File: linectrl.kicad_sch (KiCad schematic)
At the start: 22 parts, among them K1 Relay_SPST-NO, K2 Relay_SPDT, Q1 PMOS, Q2 PMOS, T1 Transformer_1P_1S, U5 LM358

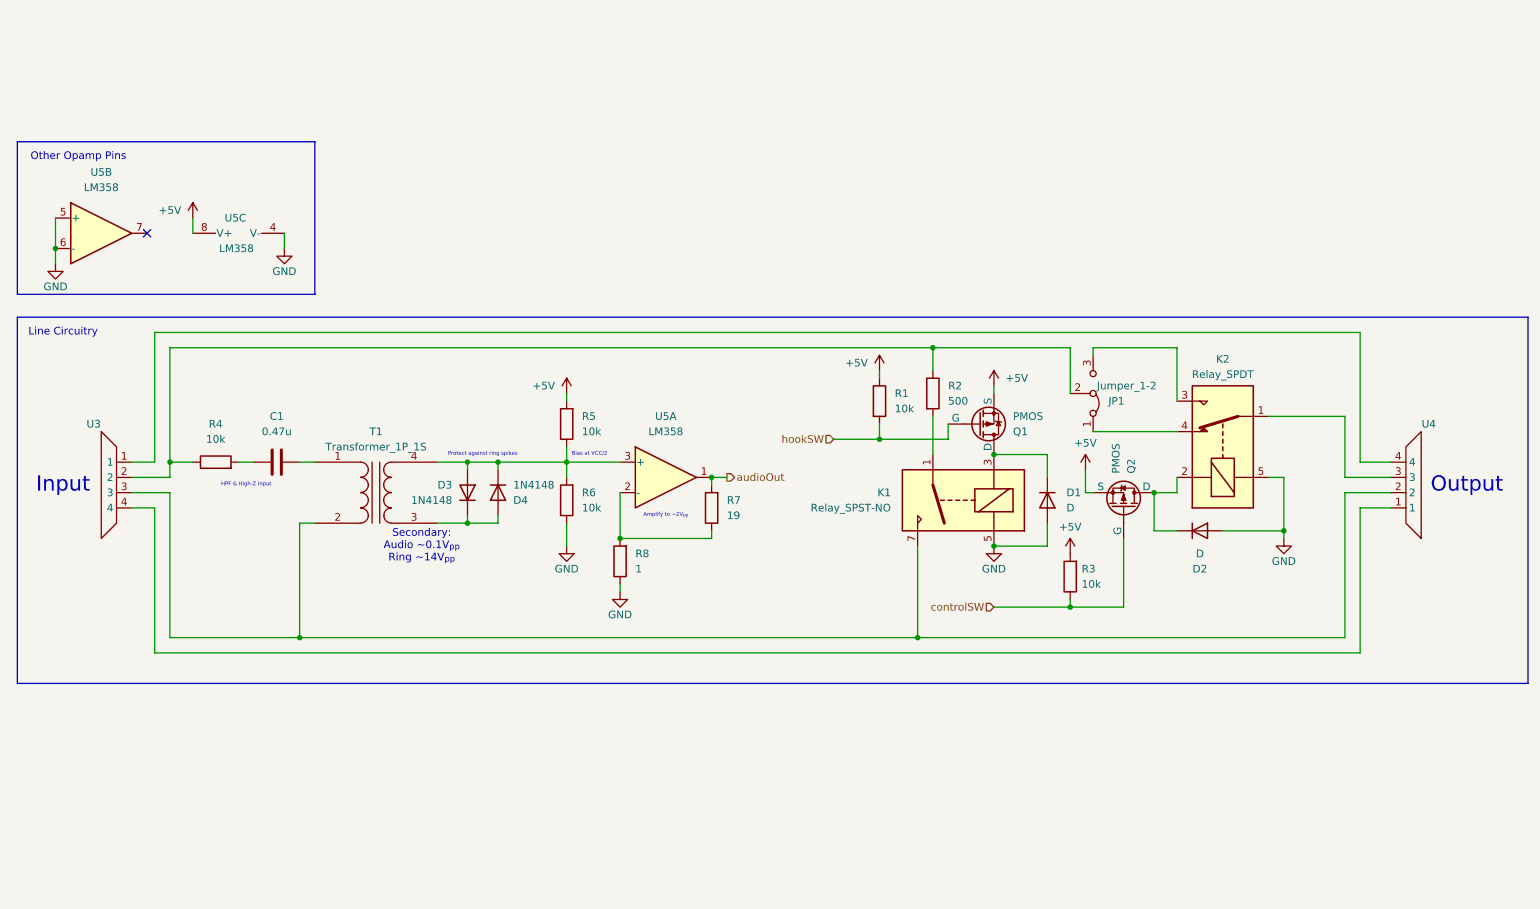
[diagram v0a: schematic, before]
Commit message: finish linectrl implementation
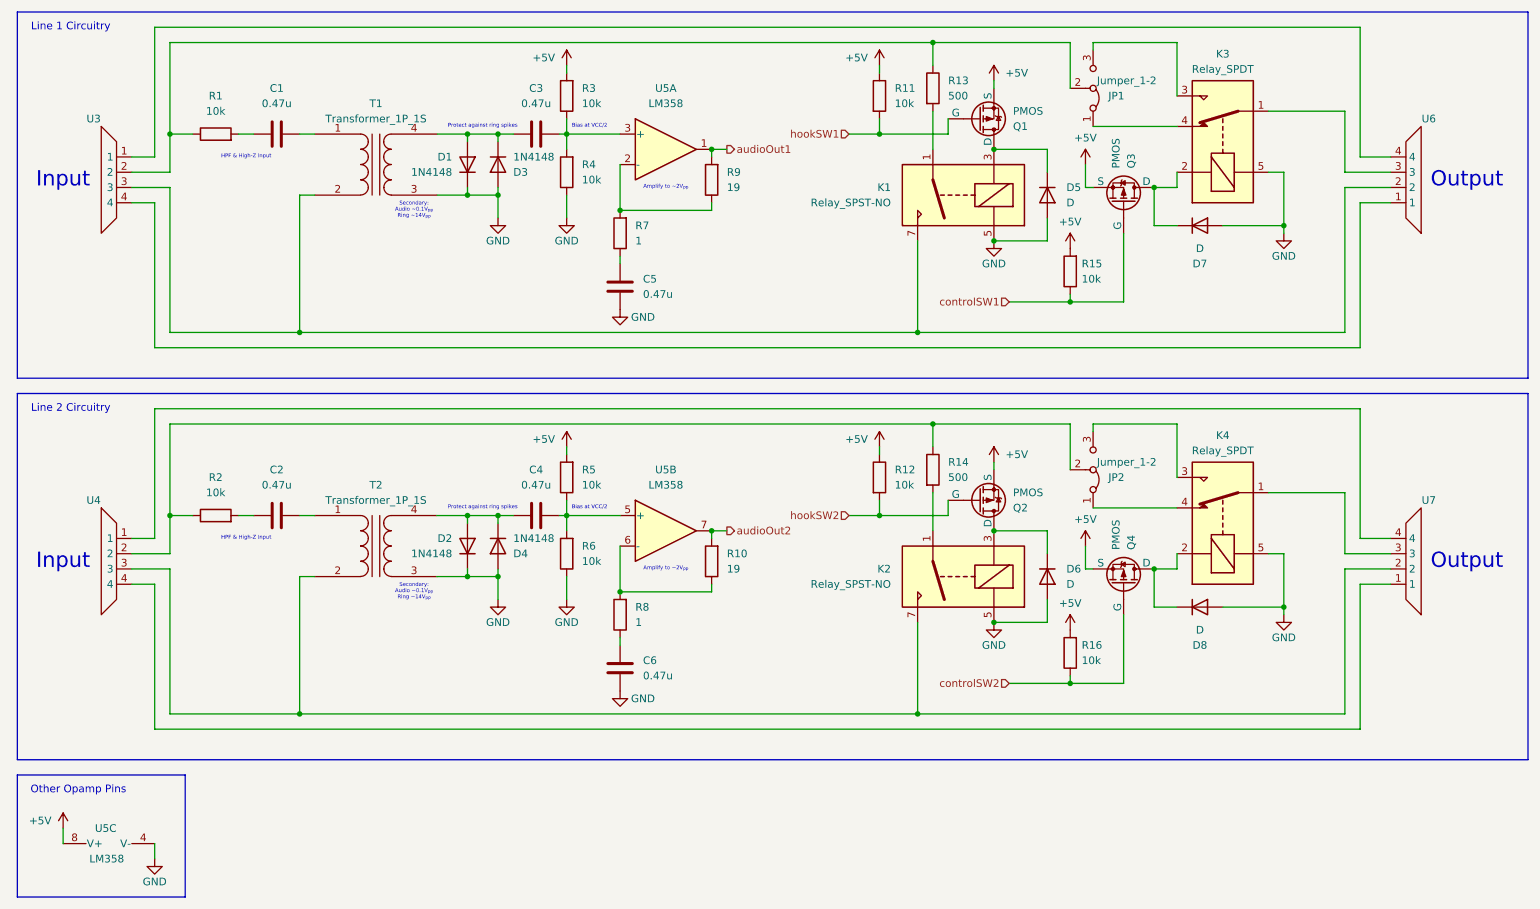
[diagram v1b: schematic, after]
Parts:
- added C2, C3, C4, C5, C6: 0.47u, symbol Device:C
- added D2, D4: 1N4148, Diode_THT:D_DO-35_SOD27_P7.62mm_Horizontal, symbol Diode:1N4148
- added D6, D8: D, Diode_THT:D_A-405_P12.70mm_Horizontal, symbol Device:D
- added JP2: Jumper_1-2, Jumper:SolderJumper-3_P1.3mm_Bridged2Bar12_RoundedPad1.0x1.5mm, symbol Jumper:Jumper_3_Bridged12
- added K2: Relay_SPST-NO, Relay_THT:Relay_SPST_StandexMeder_SIL_Form1A, symbol Relay:Relay_SPST-NO
- added K4: Relay_SPDT, Phones:K_AZ943-1C_AMZ, symbol Relay:Relay_SPDT
- added Q2, Q4: PMOS, Package_TO_SOT_THT:TO-92_HandSolder, symbol Simulation_SPICE:PMOS
- added R10: 19, symbol Device:R
- added R12, R16: 10k, Resistor_THT:R_Axial_DIN0207_L6.3mm_D2.5mm_P10.16mm_Horizontal, symbol Device:R
- added R14: 500, Resistor_THT:R_Axial_DIN0207_L6.3mm_D2.5mm_P10.16mm_Horizontal, symbol Device:R
- added R2, R5, R6: 10k, symbol Device:R
- added R8: 1, symbol Device:R
- added T2: Transformer_1P_1S, symbol Device:Transformer_1P_1S
- added U4, U7: (no value), symbol Phones:4C_Connector
- renumbered D3 to D1, D4 to D3, D1 to D5, D2 to D7, K2 to K3, Q2 to Q3, R4 to R1, R1 to R11, R2 to R13, R3 to R15, R5 to R3, R6 to R4, R8 to R7, R7 to R9, U4 to U6
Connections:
- net +5V: now also Q2.3 (S), Q4.3 (S), R12.1, R16.2, R5.2
- net GND: now also D1.1 (K), D3.2 (A), T1.3 (SA), C5.1, C6.1, D2.1 (K), D4.2 (A), D6.2 (A), D8.2 (A), K2.5, K4.5, R6.1, T2.3 (SA); no longer R7.1, U5.5 (+), U5.6 (-)
- net audioOut2: now reaches U5.7
- net audioOut2: now also R10.2
- net at D1.2 (A), D3.1 (K), T1.4 (SB): now also C3.1; no longer R3.1, R4.2, U5.3 (+)
- net audioOut renamed audioOut1
- net controlSW renamed controlSW1
- net hookSW renamed hookSW1
- new net: JP2.2 (C), R14.1, R2.1, U4.2
- new net: C2.1, R2.2
- new net: C4.2, R5.1, R6.2, U5.5 (+)
- new net: R10.1, R8.2, U5.6 (-)
- new net: JP2.1 (A), K4.4
- new net: JP2.3 (B), K4.3
- new net: K2.1, R14.2
- new net: D6.1 (K), K2.3, Q2.1 (D)
- new net: K2.7, T2.2 (AB), U4.3, U7.2
- new net: C2.2, T2.1 (AA)
- new net: C4.1, D2.2 (A), D4.1 (K), T2.4 (SB)
- new net: C6.2, R8.1
- new net: D8.1 (K), K4.2, Q4.1 (D)
- new net: C5.2, R7.1
- new net: C3.2, R3.1, R4.2, U5.3 (+)
- new net: U4.4, U7.1
- new net: K4.1, U7.3
- new net: U4.1, U7.4
- new net controlSW2: Q4.2 (G), R16.1
- new net hookSW2: Q2.2 (G), R12.2
- no-connect marks 1 -> 0
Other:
- note added: "Line 1 Circuitry"
- note added: "Line 2 Circuitry"
- note removed: "Line Circuitry"
- moved on the sheet: C1, D1, D3, D5, D7, JP1, K1, K3, Q1, Q3, R1, R11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
